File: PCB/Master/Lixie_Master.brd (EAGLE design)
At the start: 20 x 43.6 mm, 9 parts, among them IC1 FT232RL, J1 65100516121, U1 ATTINY406-MFR

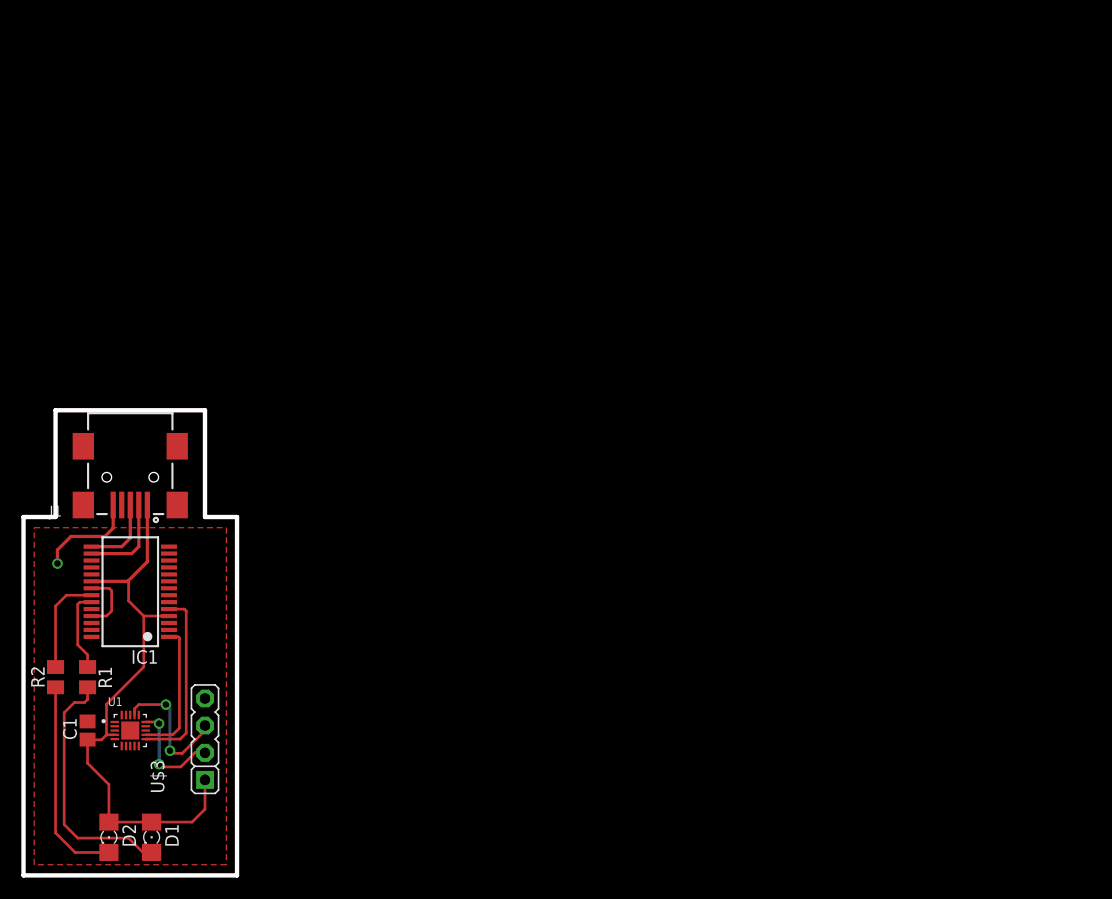
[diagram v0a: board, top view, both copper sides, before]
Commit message: V04
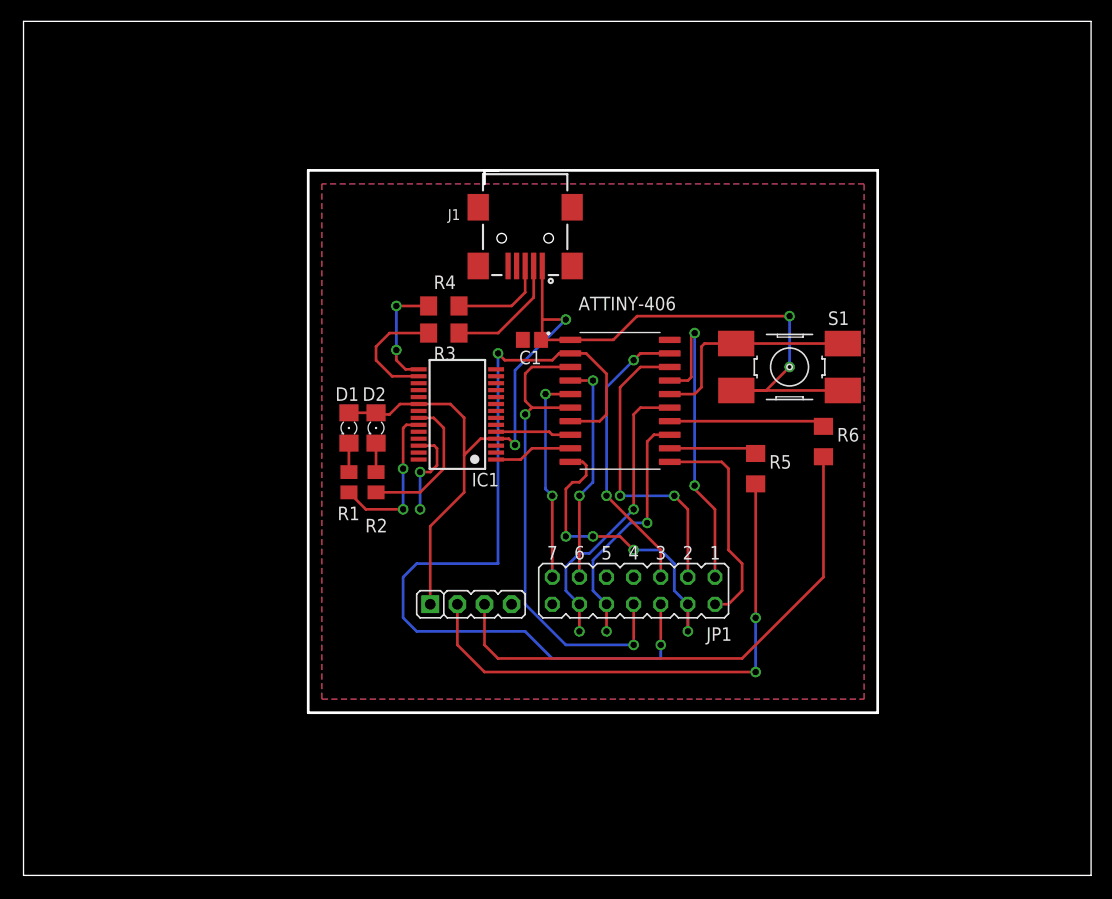
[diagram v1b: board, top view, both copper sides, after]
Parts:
- removed U1: ATTINY406-MFR, ATTINY406-MFR:QFN40P300X300X90-21N
- added ATTINY-406: (no value), SOIC127P1032X265-20N:SOIC127P1032X265-20N
- added JP1: (no value), jumper:JP7Q
- added R3, R4: 27R, 0_HTL_analog:R1206
- added R5, R6: 330R, 0_HTL_analog:R1206
- added S1: TASTER_SMD, 0_HTL_MegaCard_V3:TASTER_SMD
- moved C1 55.4 mm to (47.6, 50.2), turned to 180 degrees
- moved D2 45.8 mm to (33.0, 41.9)
- moved J1 43.2 mm to (47.0, 61.0)
- moved D1 42.6 mm to (30.5, 41.9)
- moved R2 35.1 mm to (33.0, 36.8), turned to 270 degrees
- moved IC1 34.9 mm to (40.6, 43.2)
- moved R1 30.5 mm to (30.5, 36.8), turned to 90 degrees
- moved U$3 30.0 mm to (45.7, 25.4), turned to 0 degrees
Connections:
- removed net EXP: U1.21
- new net N$10: IC1.15, R4.1
- new net N$11: ATTINY-406.16, S1.3, S1.4
- new net N$12: R5.2, U$3.2
- new net N$13: R6.2, U$3.3
- new net N$4: J1.2, R3.2
- new net PA1: ATTINY-406.17, JP1.1
- new net PA2: ATTINY-406.18, JP1.3
- new net PA3: ATTINY-406.19, JP1.5
- new net PA4: JP1.7
- new net PA5: JP1.9
- new net PA6: ATTINY-406.4, JP1.11
- new net PA7: ATTINY-406.5, JP1.13
- new net PB0: ATTINY-406.11, JP1.2
- new net PB1: ATTINY-406.10, JP1.4
- new net PB4: ATTINY-406.2, ATTINY-406.7, JP1.6
- new net PB5: ATTINY-406.3, ATTINY-406.6, JP1.8
- new net PC1: ATTINY-406.13, JP1.10
- new net PC3: ATTINY-406.15, JP1.12
- net GND: now also ATTINY-406.20, JP1.14; no longer U1.3
- net N$1: now also R4.2; no longer IC1.15
- net N$2: now also R3.1; no longer J1.2
- net N$8: now also ATTINY-406.12, R5.1; no longer U$3.2, U1.15
- net N$9: now also ATTINY-406.14, R6.1; no longer U$3.3, U1.17
- net RXD: now also ATTINY-406.9, IC1.1; no longer IC1.5, U1.11
- net TXD: now also ATTINY-406.8, IC1.5; no longer IC1.1, U1.12
- net VCC: now also ATTINY-406.1, S1.1, S1.2; no longer U1.4
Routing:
- net PB4: track 0.00 -> 82.6 mm, vias 0 -> 2
- net VCC: track 53.7 -> 104.3 mm, vias 0 -> 4
- net N$13: track 0.00 -> 50.5 mm
- net N$12: track 0.00 -> 50.4 mm, vias 0 -> 2
- net PB5: track 0.00 -> 45.8 mm, vias 0 -> 2
- net PB1: track 0.00 -> 30.1 mm, vias 0 -> 4
- net PA1: track 0.00 -> 30.1 mm, vias 0 -> 2
- net PA2: track 0.00 -> 28.8 mm, vias 0 -> 2
- net PC3: track 0.00 -> 27.7 mm, vias 0 -> 2
- net PA3: track 0.00 -> 27.1 mm, vias 0 -> 2
- net PC1: track 0.00 -> 23.7 mm, vias 0 -> 2
- net PA6: track 0.00 -> 21.1 mm, vias 0 -> 2
- net N$5: track 23.6 -> 2.71 mm
- net PB0: track 0.00 -> 20.8 mm
- net N$11: track 0.00 -> 20.4 mm
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- added copper zone on layer 16, net GND
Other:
- board size 20 x 43.6 mm -> 100 x 80 mm

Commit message: Master
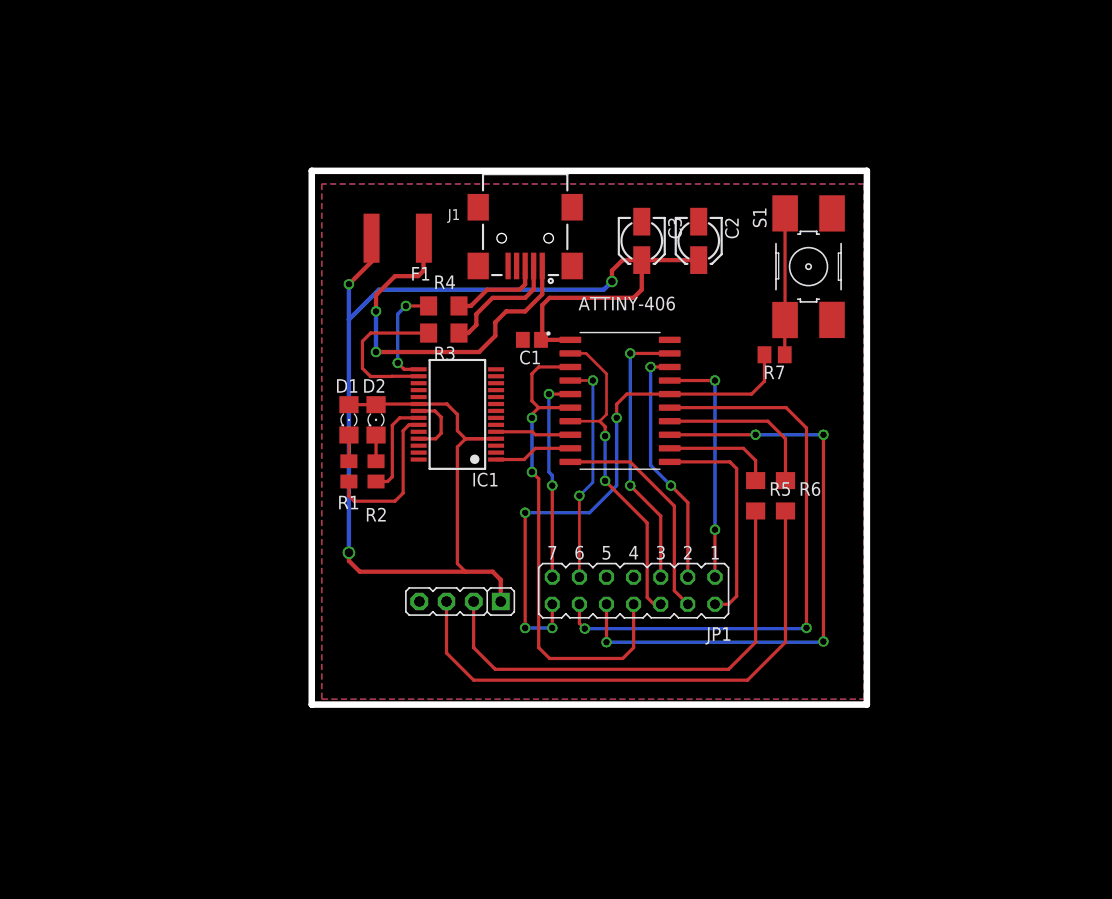
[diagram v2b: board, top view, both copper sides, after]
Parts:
- added C2, C3: 4u7, rcl:153CLV-0405
- added F1: MF-SMDF200, fuse:MF-SMDF050
- added R7: 330, 0_HTL_analog:R0805
- moved S1 9.56 mm to (73.5, 57.0), turned to 270 degrees
- moved U$3 8.64 mm to (37.1, 25.7), turned to 180 degrees
- moved R6 6.20 mm to (71.4, 35.6)
- moved R5 2.54 mm to (68.6, 35.6)
- moved R1 1.02 mm to (30.5, 37.8)
- moved R2 1.02 mm to (33.0, 37.8)
- moved D1 0.76 mm to (30.5, 42.7)
- moved D2 0.76 mm to (33.0, 42.7)
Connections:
- new net N$14: F1.1, J1.1
- new net UPDI: ATTINY-406.16, JP1.14, R7.2
- net GND: now also C2.-, C3.-, S1.1, S1.2; no longer JP1.14
- net N$11: now also R7.1; no longer ATTINY-406.16
- net VCC: now also C2.+, C3.+, F1.2; no longer J1.1, S1.1, S1.2
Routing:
- net PB4: track 82.6 -> 31.5 mm
- net UPDI: track 0.00 -> 50.0 mm, vias 0 -> 4
- net N$14: track 0.00 -> 35.0 mm, vias 0 -> 2
- net PC1: track 23.7 -> 57.7 mm, vias 2 -> 4
- net VCC: track 104.3 -> 134.8 mm, vias 4 -> 3
- net PC3: track 27.7 -> 55.6 mm
- net PB1: track 30.1 -> 21.2 mm, vias 4 -> 0
- net PA1: track 30.1 -> 22.6 mm
- net N$11: track 20.4 -> 13.3 mm
- net PA2: track 28.8 -> 22.9 mm
- net N$12: track 50.4 -> 44.9 mm, vias 2 -> 0
- net N$6: track 13.8 -> 9.29 mm
- net N$2: track 11.3 -> 14.6 mm
- net GND: track 8.75 -> 6.18 mm, vias 2 -> 0
- net N$8: track 8.25 -> 10.4 mm
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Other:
- board size 100 x 80 mm -> 52 x 50 mm
